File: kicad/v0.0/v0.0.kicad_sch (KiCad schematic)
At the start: 35 parts, among them J1 BUTTON, J2 9V_IN, J3 ESP8266_left, J4 ESP8266_right, J5 LED, J6 MOTOR, Q1 IRF520, Q2 IRF520, U2 MAX14872ETC+, U3 NE555D, U4 LM2596S-5

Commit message: finally found some pot
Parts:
- RV1: footprint (none) -> Potentiometer_THT:Potentiometer_Bourns_3296W_Vertical
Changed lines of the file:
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@@
     (property "Reference" "RV1" (id 0) (at 45.72 133.35 90))
     (property "Value" "100k" (id 1) (at 45.72 135.89 90))
-    (property "Footprint" "" (id 2) (at 45.72 139.7 0)
+    (property "Footprint" "Potentiometer_THT:Potentiometer_Bourns_3296W_Vertical" (id 2) (at 45.72 139.7 0)
       (effects (font (size 1.27 1.27)) hide)
     )
@@
     )
     (path "/0453f108-7dce-491b-878b-92849be18fad"
-      (reference "RV1") (unit 1) (value "100k") (footprint "")
+      (reference "RV1") (unit 1) (value "100k") (footprint "Potentiometer_THT:Potentiometer_Bourns_3296W_Vertical")
     )
     (path "/20935cf2-ab8a-474f-bf12-ce3a5ccf7d28"

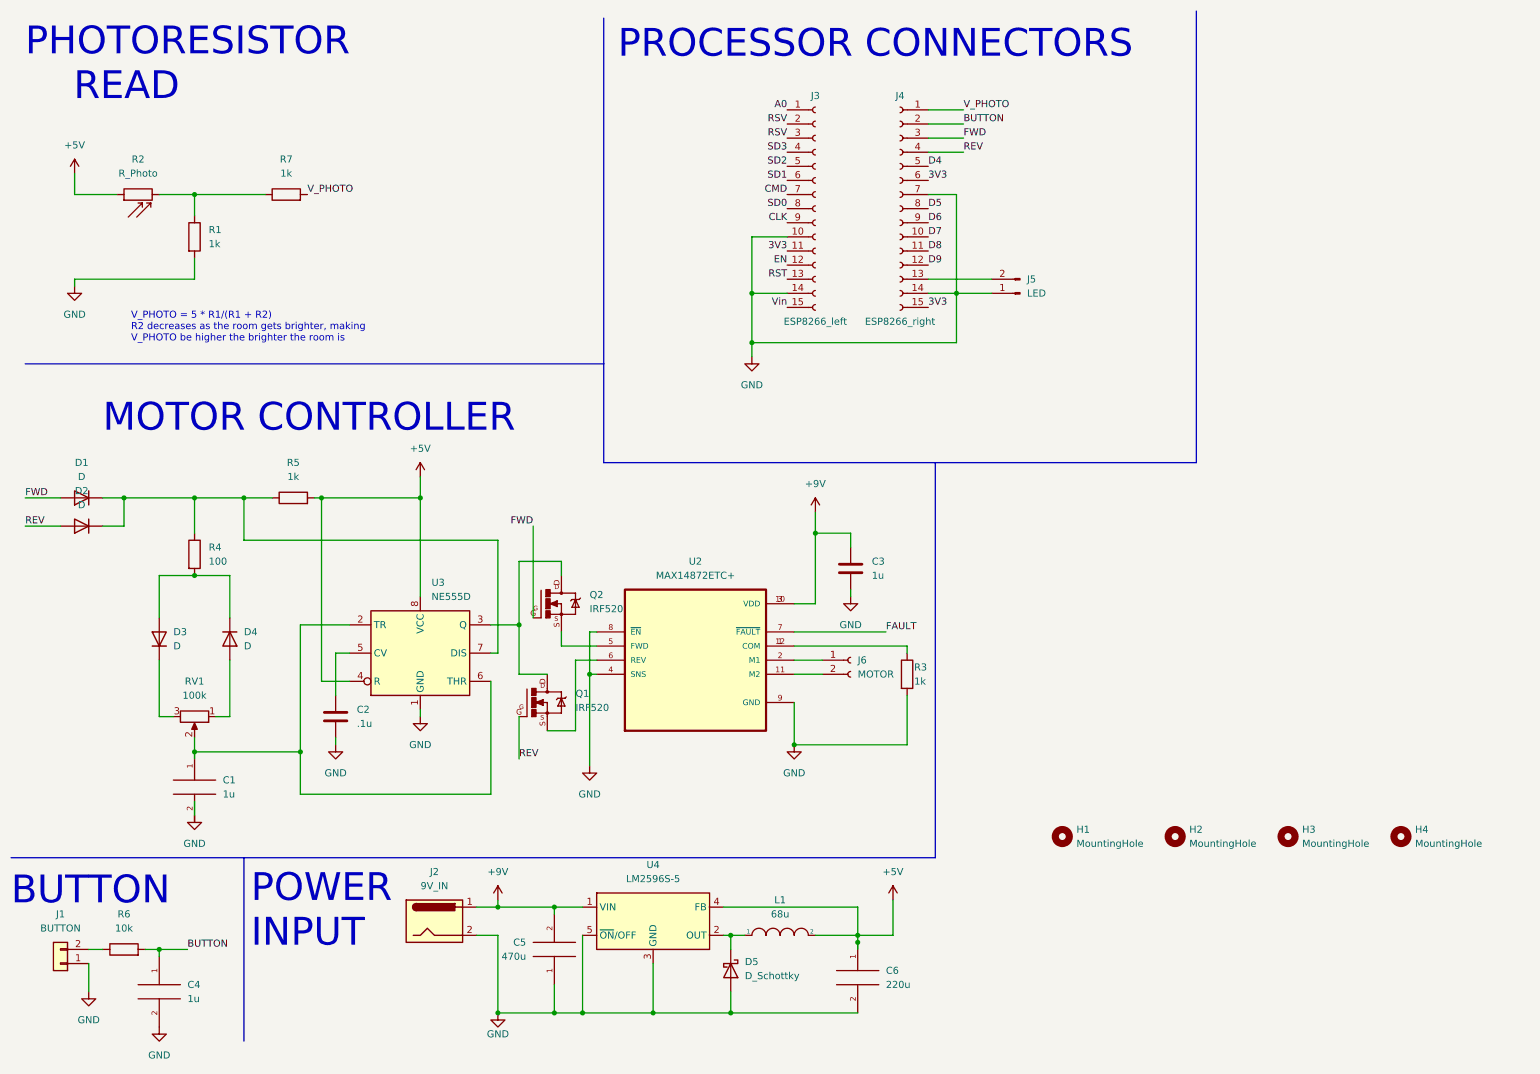
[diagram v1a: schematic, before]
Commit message: shes a beaut
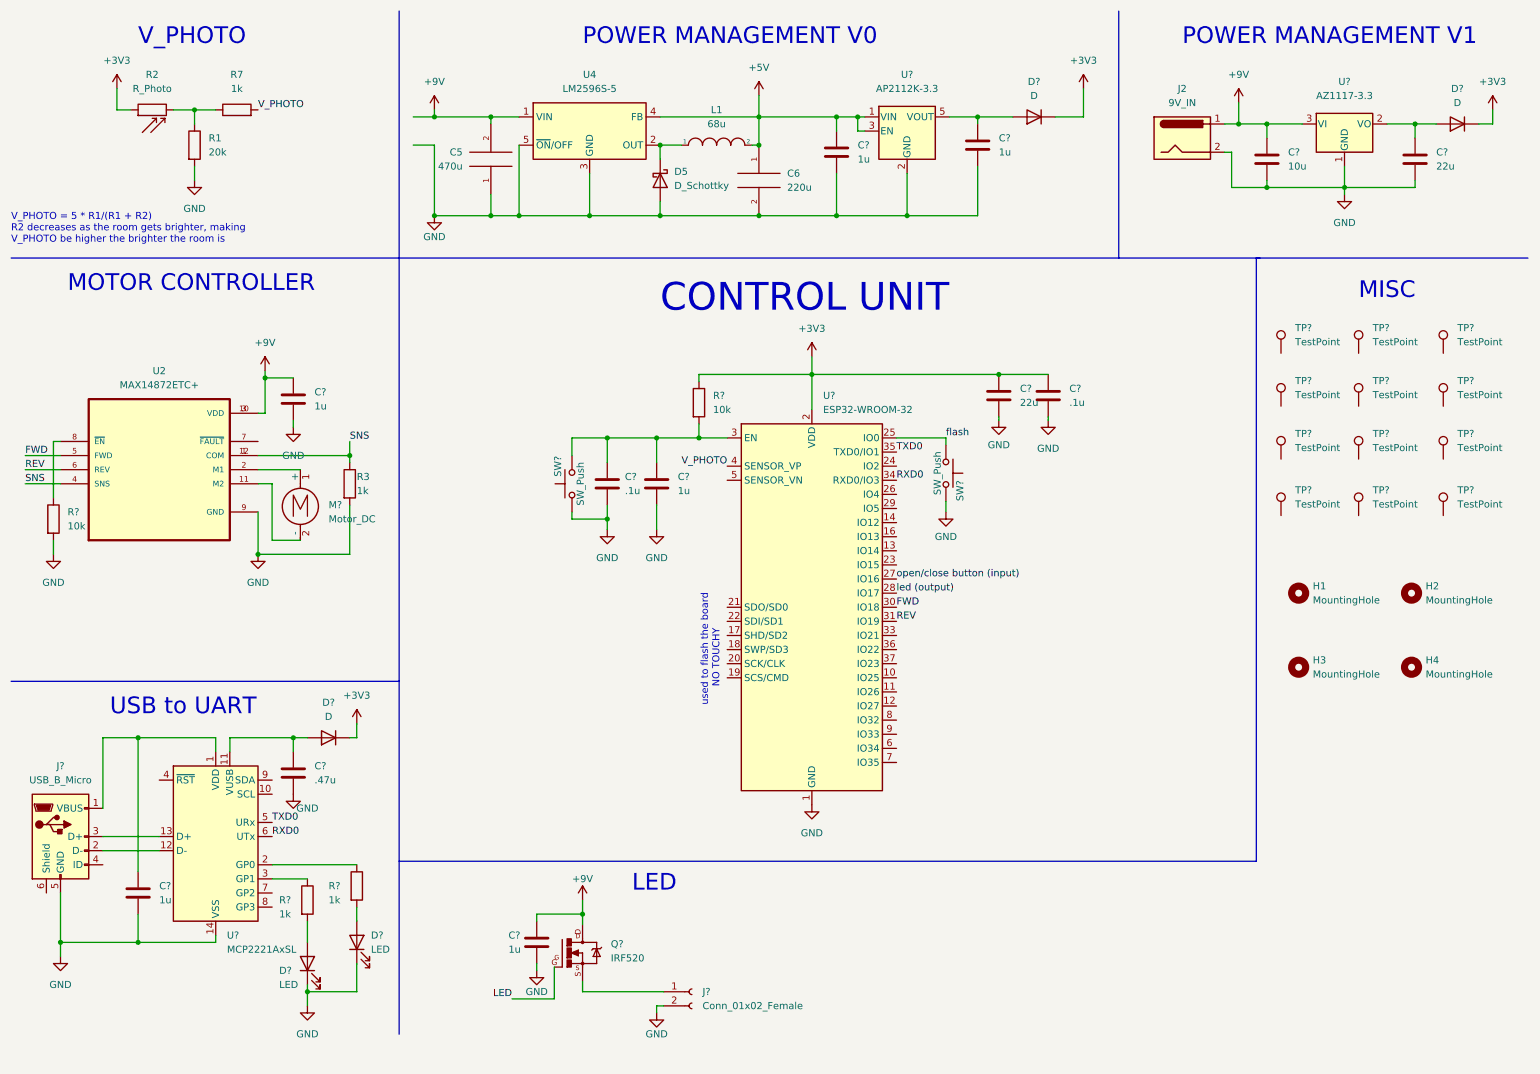
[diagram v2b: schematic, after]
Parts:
- removed C1, C4: 1u, Capacitor_SMD:C_0201_0603Metric_Pad0.64x0.40mm_HandSolder, symbol pspice:C
- removed C2: .1u, Capacitor_SMD:C_01005_0402Metric_Pad0.57x0.30mm_HandSolder, symbol Device:C
- removed C3: 1u, Capacitor_SMD:C_0201_0603Metric_Pad0.64x0.40mm_HandSolder, symbol Device:C
- removed D1, D2, D3, D4: D, Diode_SMD:D_SMA_Handsoldering, symbol Device:D
- removed J1: BUTTON, Connector_Molex:Molex_KK-254_AE-6410-02A_1x02_P2.54mm_Vertical, symbol Connector_Generic:Conn_01x02
- removed J3: ESP8266_left, Connector_PinSocket_2.54mm:PinSocket_1x15_P2.54mm_Vertical, symbol Connector:Conn_01x15_Female
- removed J4: ESP8266_right, Connector_PinSocket_2.54mm:PinSocket_1x15_P2.54mm_Vertical, symbol Connector:Conn_01x15_Female
- removed J5: LED, Connector_PinSocket_2.54mm:PinSocket_1x02_P2.54mm_Horizontal, symbol Connector:Conn_01x02_Male
- removed J6: MOTOR, Connector_PinSocket_2.54mm:PinSocket_1x02_P2.54mm_Horizontal, symbol Connector:Conn_01x02_Female
- removed Q1, Q2: IRF520, TO220BV, symbol IRF520:IRF520
- removed R4: 100, Resistor_SMD:R_0603_1608Metric_Pad0.98x0.95mm_HandSolder, symbol Device:R
- removed R5: 1k, Resistor_SMD:R_0603_1608Metric_Pad0.98x0.95mm_HandSolder, symbol Device:R
- removed R6: 10k, Resistor_SMD:R_0201_0603Metric_Pad0.64x0.40mm_HandSolder, symbol Device:R
- removed RV1: 100k, Potentiometer_THT:Potentiometer_Bourns_3296W_Vertical, symbol Device:R_Potentiometer
- removed U3: NE555D, Package_SO:SOIC-8_3.9x4.9mm_P1.27mm, symbol Timer:NE555D
- added C? (x6): 1u, symbol Device:C
- added C? (x2): 22u, symbol Device:C
- added C? (x2): .1u, symbol Device:C
- added C?: .47u, symbol Device:C
- added C?: 10u, symbol Device:C
- added D? (x3): D, symbol Device:D
- added D? (x2): LED, symbol Device:LED
- added J?: USB_B_Micro, symbol Connector:USB_B_Micro
- added J?: Conn_01x02_Female, symbol Connector:Conn_01x02_Female
- added M?: Motor_DC, symbol Motor:Motor_DC
- added Q?: IRF520, TO220BV, symbol IRF520:IRF520
- added R? (x2): 10k, symbol Device:R
- added R? (x2): 1k, symbol Device:R
- added SW? (x2): SW_Push, symbol Switch:SW_Push
- added TP? (x12): TestPoint, symbol Connector:TestPoint
- added U?: AZ1117-3.3, symbol Regulator_Linear:AZ1117-3.3
- added U?: MCP2221AxSL, Package_SO:SOIC-14_3.9x8.7mm_P1.27mm, symbol Interface_USB:MCP2221AxSL
- added U?: AP2112K-3.3, Package_TO_SOT_SMD:SOT-23-5, symbol Regulator_Linear:AP2112K-3.3
- added U?: ESP32-WROOM-32, RF_Module:ESP32-WROOM-32, symbol RF_Module:ESP32-WROOM-32
- R1: value 1k -> 20k
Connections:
- net +5V: now also C?.1, U?.1 (VIN), U?.3 (EN); no longer R2.1
- net +9V: now also C?.1, C?.1, C?.1, Q?.D, U?.3 (VI)
- net FWD: now also U2.5 (FWD), U?.30 (IO18)
- net GND: now also C?.2, C?.2, C?.2, C?.2, C?.2, C?.2, C?.2, C?.2, C?.2, C?.2, C?.2, C?.2, D?.1 (K), D?.1 (K), J?.2 (Pin_2), J?.5 (GND), R?.2, SW?.1, SW?.2, U?.1 (GND), U?.1 (GND), U?.14 (VSS), U?.15 (GND), U?.2 (GND), U?.38 (GND), U?.39 (GND); no longer U2.4 (SNS), U2.8 (~{EN})
- net REV: now also U2.6 (REV), U?.31 (IO19)
- net V_PHOTO: now also U?.4 (SENSOR_VP)
- net SNS: now reaches R3.1, U2.1 (COM), U2.12 (COM)
- net SNS: now also U2.4 (SNS)
- net at U2.11 (M2): now also M?.2 (-)
- net at U2.2 (M1): now also M?.1 (+)
- net FAULT: no longer names the net of U2.7 (~{FAULT})
- new net: C?.1, D?.2 (A), U?.2 (VO)
- new net: C?.1, J?.1 (VBUS), U?.1 (VDD)
- new net: C?.1, D?.2 (A), U?.5 (VOUT)
- new net: R?.1, U2.8 (~{EN})
- new net: C?.1, C?.1, R?.2, SW?.2, U?.3 (EN)
- new net: R?.1, U?.3 (GP1)
- new net: D?.2 (A), R?.2 (x2)
- new net: C?.1, D?.2 (A), U?.11 (VUSB)
- new net: J?.2 (D-), U?.12 (D-)
- new net: J?.3 (D+), U?.13 (D+)
- new net: R?.1, U?.2 (GP0)
- new net: J?.1 (Pin_1), Q?.S
- new net +3V3: C?.1, C?.1, D?.1 (K), D?.1 (K), D?.1 (K), R2.1, R?.1, U?.2 (VDD)
- new net LED: Q?.G
- new net RXD0: U?.34 (RXD0/IO3), U?.6 (UTx)
- new net TXD0: U?.35 (TXD0/IO1), U?.5 (URx)
- new net flash: SW?.1, U?.25 (IO0)
- new net led (output): U?.28 (IO17)
- new net open/close button (input): U?.27 (IO16)
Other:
- note added: "CONTROL UNIT"
- note added: "LED"
- note added: "MISC"
- note added: "POWER MANAGEMENT V0"
- note added: "POWER MANAGEMENT V1"
- note added: "USB to UART"
- note added: "V_PHOTO"
- note added: "used to flash the board NO TOUCHY"
- note removed: "BUTTON"
- note removed: "PHOTORESISTOR READ"
- note removed: "POWER INPUT"
- note removed: "PROCESSOR CONNECTORS"
- moved on the sheet: C5, C6, D5, H1, H2, H3, H4, J2, L1, R1, R2, R3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
